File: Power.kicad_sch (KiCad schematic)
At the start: 29 parts, among them J7 Conn_01x02, J8 Conn_01x03, Q1 AO3400A, Q2 AO3401A, Q3 AO3401A, U1 TPS62130

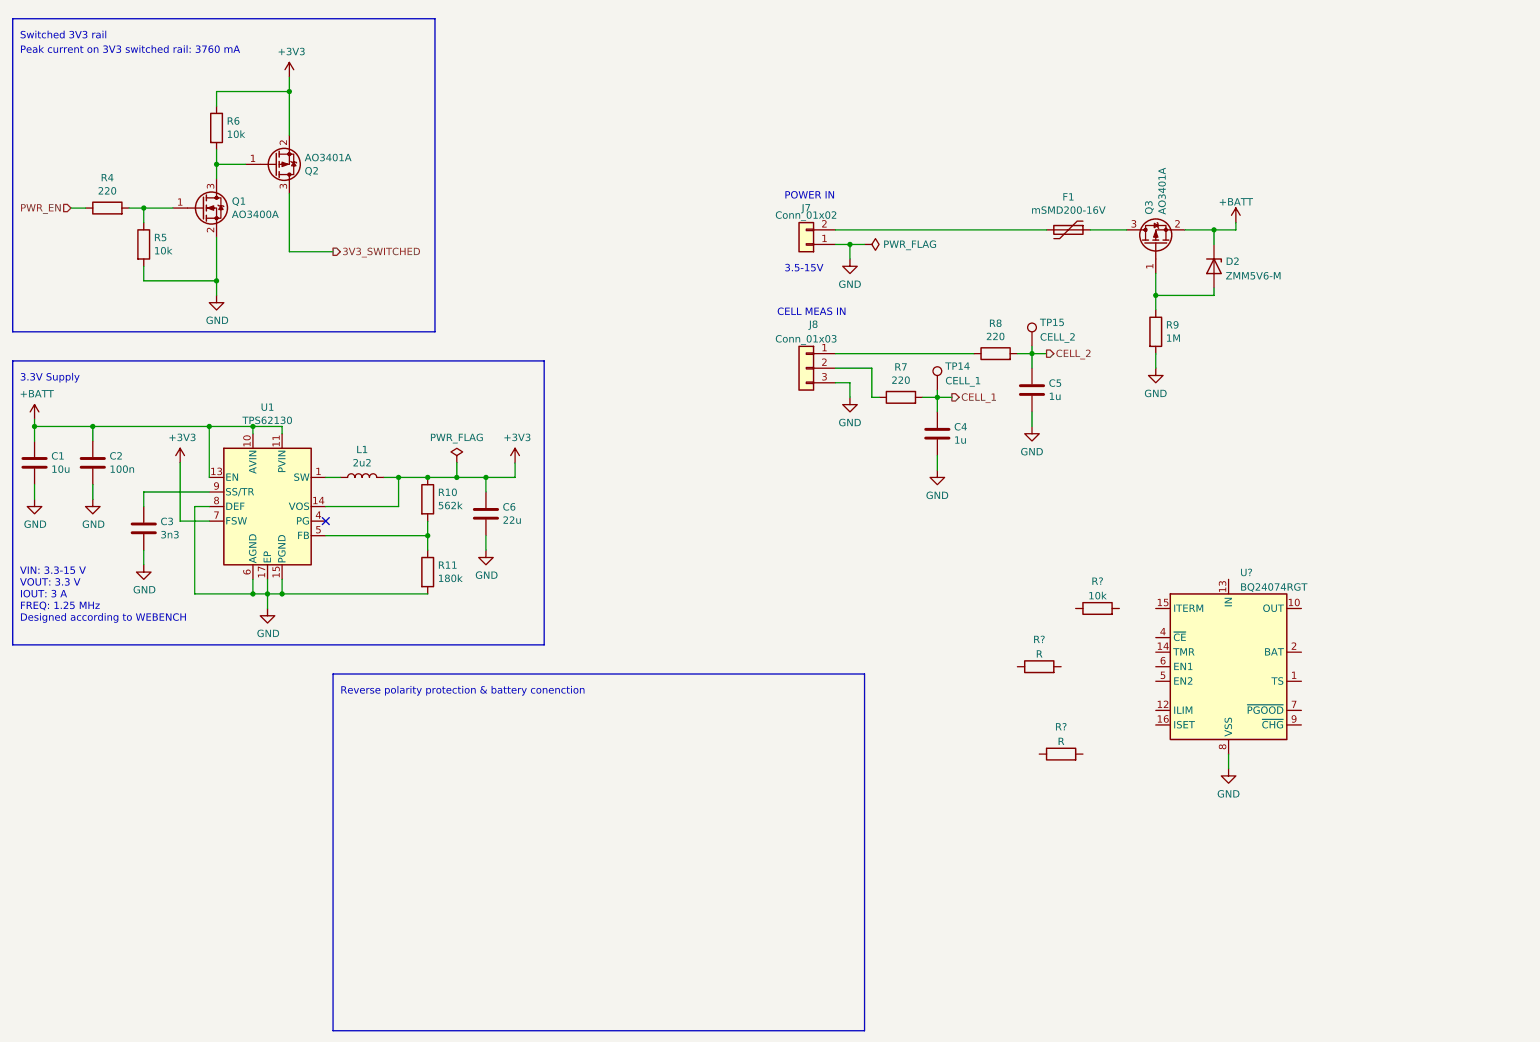
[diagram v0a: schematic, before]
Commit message: Checkpoint
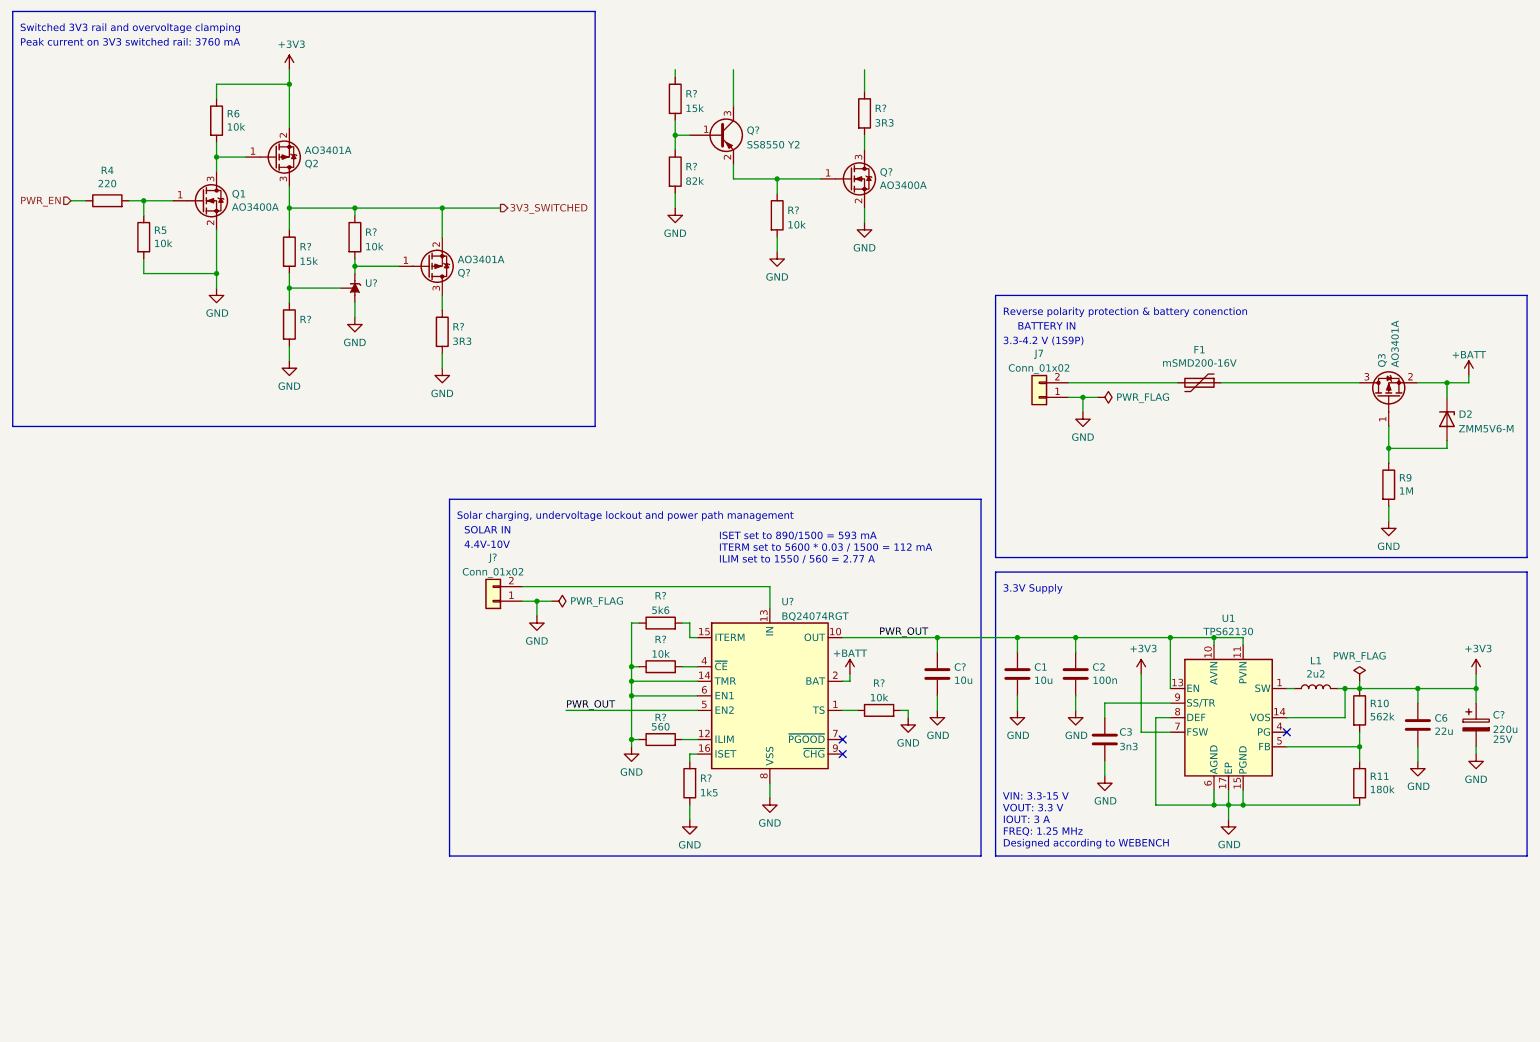
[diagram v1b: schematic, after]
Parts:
- removed C4, C5: 1u, Capacitor_SMD:C_0603_1608Metric, symbol Device:C
- removed J8: Conn_01x03, Connector_JST:JST_XH_B3B-XH-AM_1x03_P2.50mm_Vertical, symbol Connector_Generic:Conn_01x03
- removed R7, R8: 220, Resistor_SMD:R_0603_1608Metric, symbol Device:R
- removed TP14: CELL_1, TestPoint:TestPoint_Loop_D2.50mm_Drill1.0mm_LowProfile, symbol Connector:TestPoint
- removed TP15: CELL_2, TestPoint:TestPoint_Loop_D2.50mm_Drill1.0mm_LowProfile, symbol Connector:TestPoint
- added C?: 10u, Capacitor_SMD:C_0805_2012Metric, symbol Device:C
- added C?: 220u, Capacitor_THT:CP_Radial_D8.0mm_P3.50mm, symbol Device:C_Polarized
- added J?: Conn_01x02, Connector_JST:JST_XH_B2B-XH-AM_1x02_P2.50mm_Vertical, symbol Connector_Generic:Conn_01x02
- added Q?: SS8550 Y2, symbol Device:Q_PNP_BEC
- added Q?: AO3400A, Package_TO_SOT_SMD:SOT-23, symbol Transistor_FET:AO3400A
- added Q?: AO3401A, Package_TO_SOT_SMD:SOT-23, symbol Transistor_FET:AO3401A
- added R?: 1k5, symbol Device:R
- added R? (x2): 15k, symbol Device:R
- added R? (x2): 3R3, symbol Device:R
- added R? (x3): 10k, symbol Device:R
- added R?: (no value), symbol Device:R
- added R?: 82k, symbol Device:R
- added U?: (no value), symbol Reference_Voltage:TL431PK
- R?: value R -> 5k6
- R?: value R -> 560
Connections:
- net +3V3: now also C?.1
- net +BATT: now also U?.2 (BAT), U?.3 (BAT); no longer C1.1, C2.1, U1.10 (AVIN), U1.11 (PVIN), U1.12 (PVIN), U1.13 (EN)
- net 3V3_SWITCHED: now also Q?.2 (S), R?.1, R?.1
- net GND: now also R?.1, R?.1, R?.2, U?.14 (TMR), U?.6 (EN1), C?.2, C?.2, J?.1 (Pin_1), Q?.2 (S), R?.1, R?.1, R?.2, R?.2, R?.2, R?.2, U?.2 (A)
- net at R?.1: now also U?.1 (TS)
- net at R?.2: now also U?.15 (ITERM)
- net PWR_OUT: now reaches U?.10 (OUT), U?.11 (OUT)
- net PWR_OUT: now also C1.1, C2.1, U1.10 (AVIN), U1.11 (PVIN), U1.12 (PVIN), U1.13 (EN), U?.5 (EN2), C?.1
- net at U?.12 (ILIM): now also R?.2
- net at U?.13 (IN): now also J?.2 (Pin_2)
- net at U?.16 (ISET): now also R?.2
- net at U?.4 (~{CE}): now also R?.2
- new net: R?.1, R?.2, U?.1 (REF)
- new net: Q?.3 (D), R?.2
- new net: Q?.1 (G), Q?.2 (E), R?.1
- new net: Q?.1 (B), R?.1, R?.2
- new net: Q?.3 (D), R?.1
- new net: Q?.1 (G), R?.2, U?.3 (K)
- no-connect marks 1 -> 3
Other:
- note added: "3.3-4.2 V (1S9P)"
- note added: "4.4V-10V"
- note added: "BATTERY IN"
- note added: "ISET set to 890/1500 = 593 mA ITERM set to 5600 * 0.03 / 1500 = 112 mA ILIM set to 1550 / 560 = 2.77 A"
- note added: "SOLAR IN"
- note added: "Solar charging, undervoltage lockout and power path management"
- note added: "Switched 3V3 rail and overvoltage clamping"
- note removed: "3.5-15V"
- note removed: "CELL MEAS IN"
- note removed: "POWER IN"
- note removed: "Switched 3V3 rail"
- moved on the sheet: C1, C2, C3, C6, D2, F1, J7, L1, Q1, Q2, Q3, R10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
